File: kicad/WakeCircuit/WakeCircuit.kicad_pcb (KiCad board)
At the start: 2 copper layers, 58.5 x 28 mm, 15 parts, among them J1 Conn_01x12_Socket, J2 Conn_01x10_Socket, U1 TLV7011DBVR, U3 4013

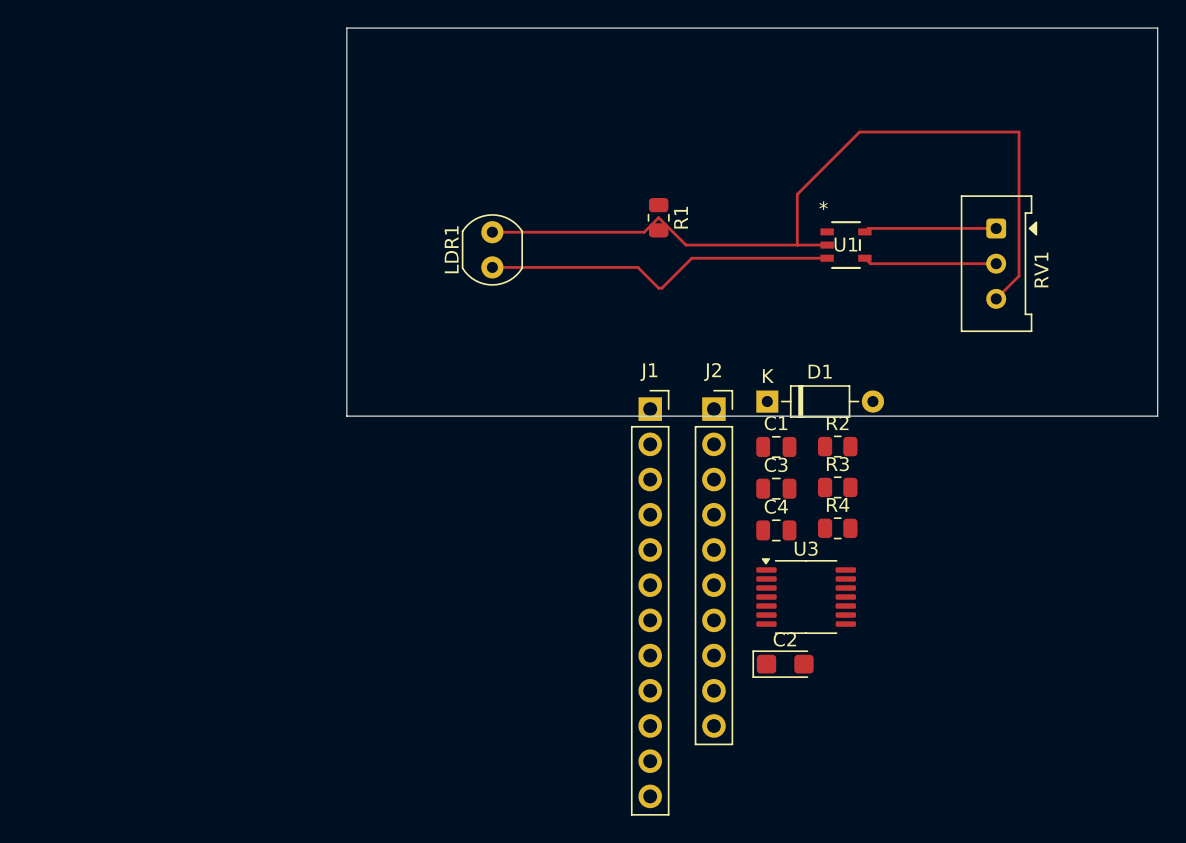
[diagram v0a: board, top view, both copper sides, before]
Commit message: PCB layout
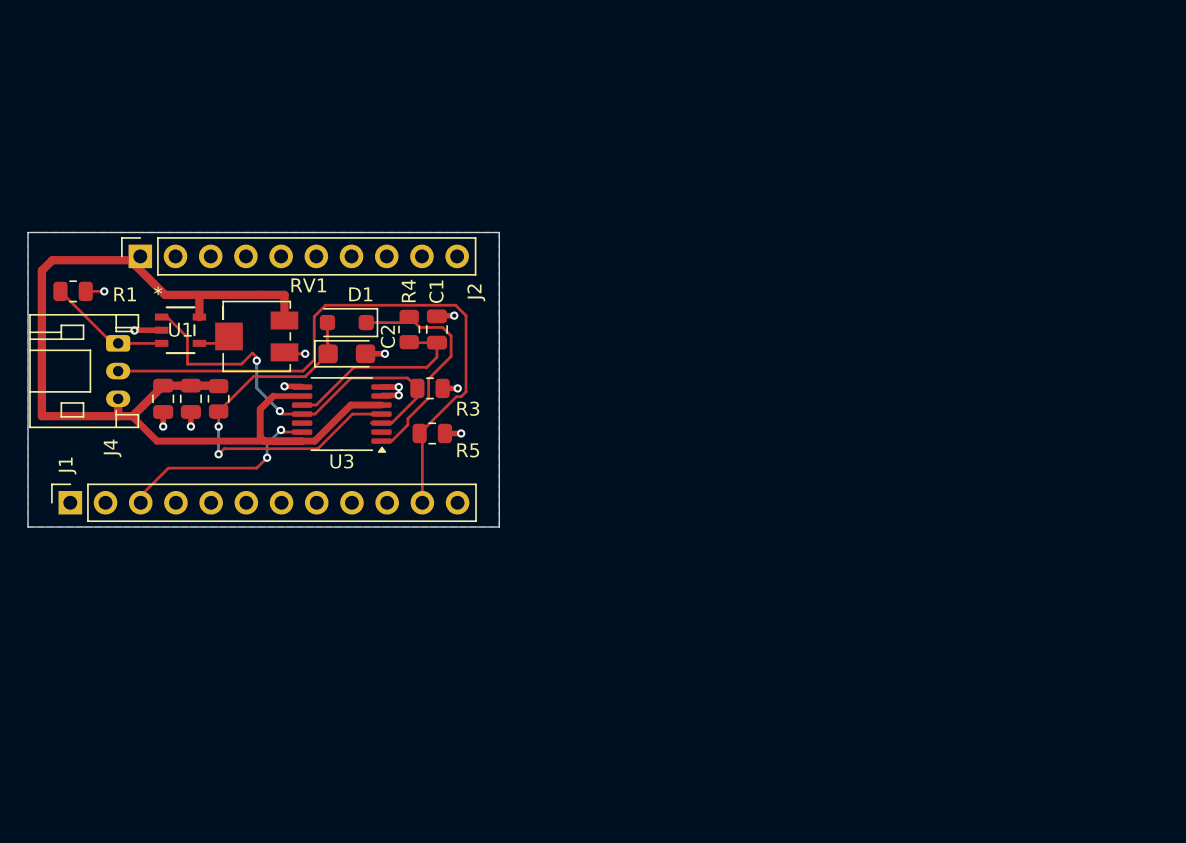
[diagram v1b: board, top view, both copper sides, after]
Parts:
- removed LDR1: GL5539, OptoDevice:R_LDR_4.9x4.2mm_P2.54mm_Vertical
- added J4: Conn_01x03_Socket, Connector_JST:JST_PH_S3B-PH-K_1x03_P2.00mm_Horizontal, F.Cu at (98.0, 104.8)
- added R5: 1.2K, Resistor_SMD:R_0805_2012Metric, F.Cu at (120.7, 111.2)
- D1: footprint Diode_THT:D_DO-35_SOD27_P7.62mm_Horizontal -> Diode_SMD:D_SOD-123F
- RV1: footprint Potentiometer_THT:Potentiometer_Bourns_3386W_Horizontal -> Potentiometer_SMD:Potentiometer_Bourns_3214J_Horizontal
- moved RV1 53.9 mm to (108.0, 104.2), turned to 0 degrees
- moved U1 48.4 mm to (102.5, 103.8)
- moved C4 45.2 mm to (101.2, 108.8), turned to 90 degrees
- moved R2 44.8 mm to (105.2, 108.8), turned to 90 degrees
- moved J2 42.8 mm to (99.6, 98.5), turned to 90 degrees
- moved C3 42.7 mm to (103.2, 108.8), turned to -90 degrees
- moved R1 42.6 mm to (94.8, 101.0), turned to 180 degrees
- moved J1 42.4 mm to (94.5, 116.2), turned to 90 degrees
- moved C2 38.8 mm to (114.5, 105.5)
- moved U3 36.0 mm to (114.1, 109.8), turned to 180 degrees
- moved R4 34.1 mm to (119.0, 103.8), turned to 90 degrees
- moved D1 30.9 mm to (114.5, 103.2), turned to 180 degrees
- moved R3 30.3 mm to (120.5, 108.0)
- moved C1 25.9 mm to (121.0, 103.8), turned to 90 degrees
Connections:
- net /ESP32 GPIO 5 Wake renamed GPIO_5
- net Net-(U1-IN+) renamed LDR_SIG
- J1 pad 11: unconnected-(J1-Pin_11-Pad11) -> GPIO_1
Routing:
- net +3V3: track 9.58 -> 76.3 mm
- net GPIO_1: track 0.00 -> 44.4 mm
- net GND: track 59.6 -> 16.0 mm, vias 0 -> 12
- net Net-(U1-OUT): track 0.00 -> 30.5 mm, vias 0 -> 2
- net Net-(D1-A): track 0.00 -> 28.4 mm, vias 0 -> 2
- net Net-(D1-K): track 0.00 -> 17.0 mm
- net LDR_SIG: track 25.7 -> 8.90 mm
- net GPIO_5: track 0.00 -> 14.4 mm, vias 0 -> 2
- net Net-(U3B-R): track 0.00 -> 14.2 mm
- net Net-(U1-IN-): track 9.64 -> 2.34 mm
- added copper zone on B.Cu, net GND
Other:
- board size 58.5 x 28 mm -> 34 x 21.2 mm
- board text added: "C2"
